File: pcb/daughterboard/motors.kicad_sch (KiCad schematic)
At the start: 20 parts, among them J10 Conn_01x06_Socket, J11 Conn_01x06_Socket, J12 Conn_01x06_Socket, J13 Conn_01x06_Socket, J14 Conn_01x06_Socket, J15 Conn_01x06_Socket, J16 Conn_01x06_Socket, J17 Conn_01x06_Socket, J18 Conn_01x06_Socket, J19 Conn_01x06_Socket, J20 Conn_01x06_Socket, J21 Conn_01x06_Socket, J22 Conn_01x06_Socket, J3 Conn_01x06_Socket, J4 Conn_01x06_Socket, J5 Conn_01x06_Socket, J6 Conn_01x06_Socket, J7 Conn_01x06_Socket, J8 Conn_01x06_Socket, J9 Conn_01x06_Socket

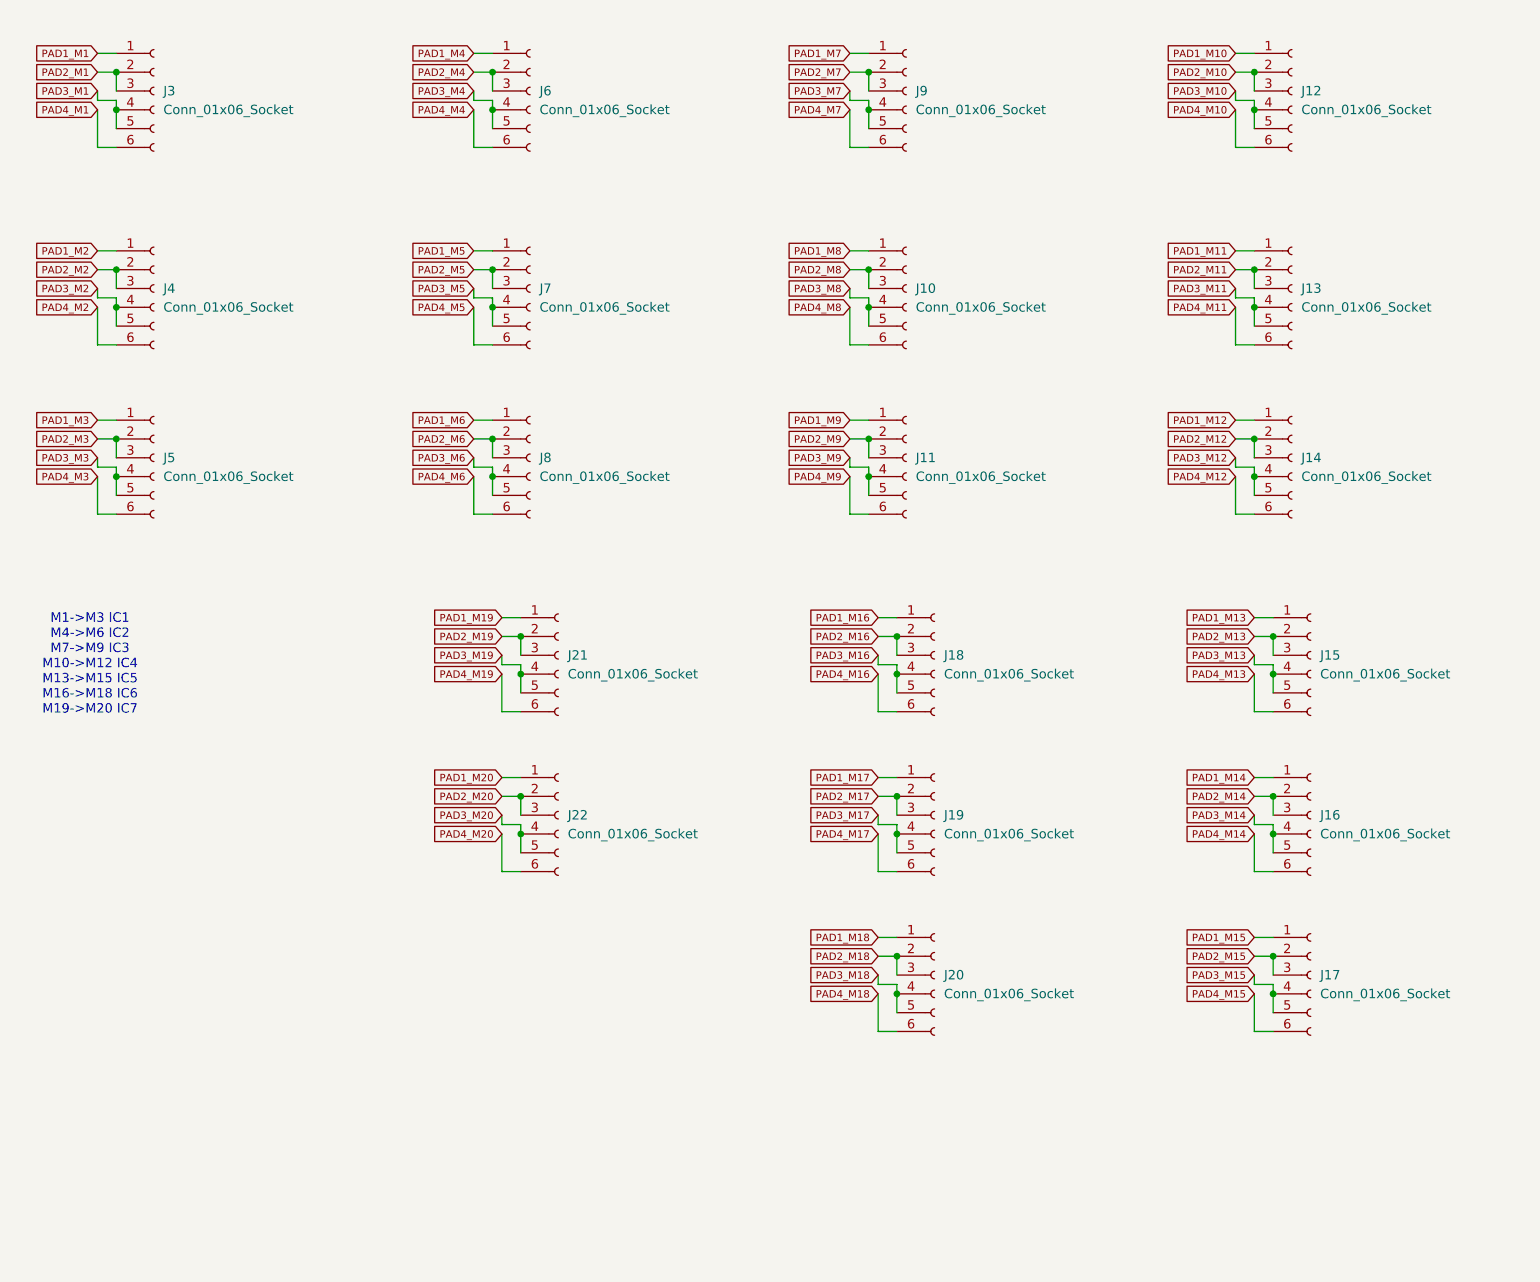
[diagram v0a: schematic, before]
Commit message: modified motor connectors
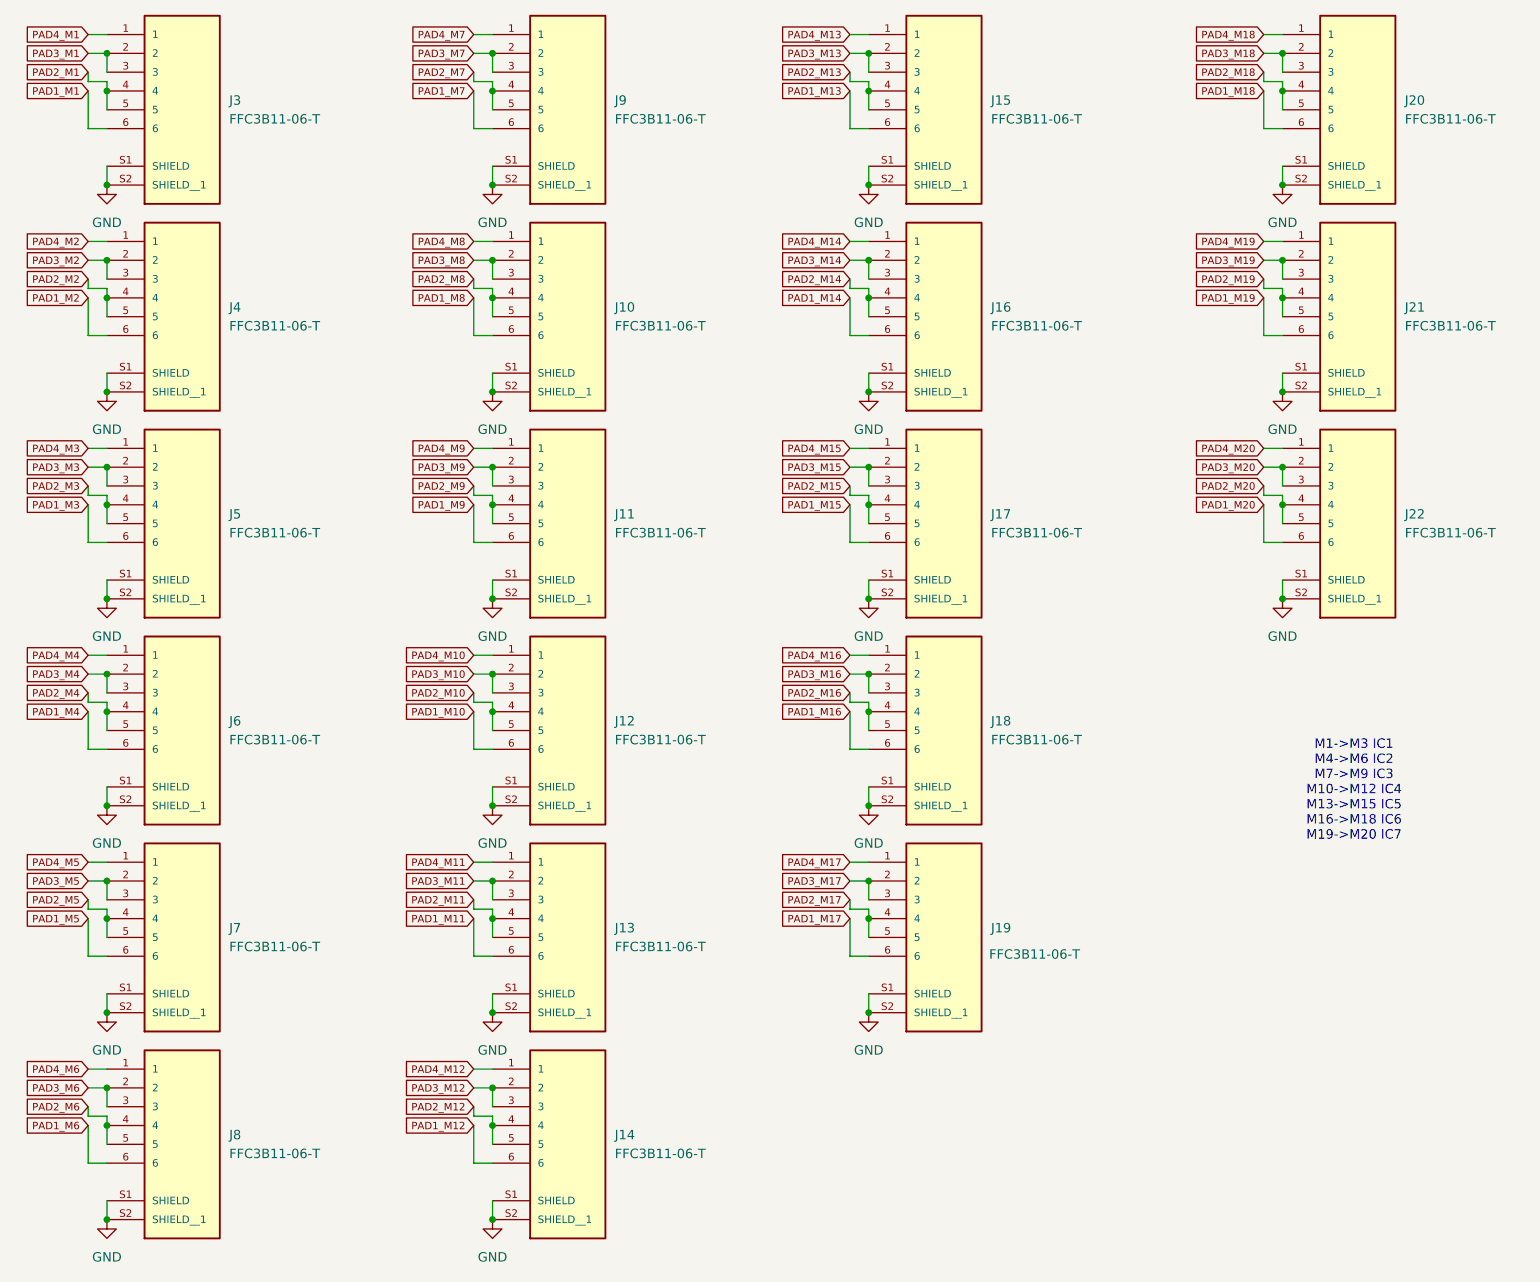
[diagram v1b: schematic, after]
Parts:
- removed J10, J11, J12, J13, J14, J15, J16, J17, J18, J19, J20, J21, J22, J3, J4, J5, J6, J7, J8, J9: Conn_01x06_Socket, 52207-0633:52207-0633, symbol Connector:Conn_01x06_Socket
- added J10, J11, J12, J13, J14, J15, J16, J17, J18, J19, J20, J21, J22, J3, J4, J5, J6, J7, J8, J9: FFC3B11-06-T, FFC3B11_06_T:GCT_FFC3B11-06-T, symbol FFC3B11-06-T:FFC3B11-06-T
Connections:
- net PAD1_M1: now also J3.6
- net PAD1_M10: now also J12.6
- net PAD1_M11: now also J13.6
- net PAD1_M12: now also J14.6
- net PAD1_M13: now also J15.6
- net PAD1_M14: now also J16.6
- net PAD1_M15: now also J17.6
- net PAD1_M16: now also J18.6
- net PAD1_M17: now also J19.6
- net PAD1_M18: now also J20.6
- net PAD1_M19: now also J21.6
- net PAD1_M2: now also J4.6
- net PAD1_M20: now also J22.6
- net PAD1_M3: now also J5.6
- net PAD1_M4: now also J6.6
- net PAD1_M5: now also J7.6
- net PAD1_M6: now also J8.6
- net PAD1_M7: now also J9.6
- net PAD1_M8: now also J10.6
- net PAD1_M9: now also J11.6
- net PAD2_M1: now also J3.4, J3.5
- net PAD2_M10: now also J12.4, J12.5
- net PAD2_M11: now also J13.4, J13.5
- net PAD2_M12: now also J14.4, J14.5
- net PAD2_M13: now also J15.4, J15.5
- net PAD2_M14: now also J16.4, J16.5
- net PAD2_M15: now also J17.4, J17.5
- net PAD2_M16: now also J18.4, J18.5
- net PAD2_M17: now also J19.4, J19.5
- net PAD2_M18: now also J20.4, J20.5
- net PAD2_M19: now also J21.4, J21.5
- net PAD2_M2: now also J4.4, J4.5
- net PAD2_M20: now also J22.4, J22.5
- net PAD2_M3: now also J5.4, J5.5
- net PAD2_M4: now also J6.4, J6.5
- net PAD2_M5: now also J7.4, J7.5
- net PAD2_M6: now also J8.4, J8.5
- net PAD2_M7: now also J9.4, J9.5
- net PAD2_M8: now also J10.4, J10.5
- net PAD2_M9: now also J11.4, J11.5
- net PAD3_M1: now also J3.2, J3.3
- net PAD3_M10: now also J12.2, J12.3
- net PAD3_M11: now also J13.2, J13.3
- net PAD3_M12: now also J14.2, J14.3
- net PAD3_M13: now also J15.2, J15.3
- net PAD3_M14: now also J16.2, J16.3
- net PAD3_M15: now also J17.2, J17.3
- net PAD3_M16: now also J18.2, J18.3
- net PAD3_M17: now also J19.2, J19.3
- net PAD3_M18: now also J20.2, J20.3
- net PAD3_M19: now also J21.2, J21.3
- net PAD3_M2: now also J4.2, J4.3
- net PAD3_M20: now also J22.2, J22.3
- net PAD3_M3: now also J5.2, J5.3
- net PAD3_M4: now also J6.2, J6.3
- net PAD3_M5: now also J7.2, J7.3
- net PAD3_M6: now also J8.2, J8.3
- net PAD3_M7: now also J9.2, J9.3
- net PAD3_M8: now also J10.2, J10.3
- net PAD3_M9: now also J11.2, J11.3
- net PAD4_M1: now also J3.1
- net PAD4_M10: now also J12.1
- net PAD4_M11: now also J13.1
- net PAD4_M12: now also J14.1
- net PAD4_M13: now also J15.1
- net PAD4_M14: now also J16.1
- net PAD4_M15: now also J17.1
- net PAD4_M16: now also J18.1
- net PAD4_M17: now also J19.1
- net PAD4_M18: now also J20.1
- net PAD4_M19: now also J21.1
- net PAD4_M2: now also J4.1
- net PAD4_M20: now also J22.1
- net PAD4_M3: now also J5.1
- net PAD4_M4: now also J6.1
- net PAD4_M5: now also J7.1
- net PAD4_M6: now also J8.1
- net PAD4_M7: now also J9.1
- net PAD4_M8: now also J10.1
- net PAD4_M9: now also J11.1
- new net GND: J10.S1 (SHIELD), J10.S2 (SHIELD__1), J11.S1 (SHIELD), J11.S2 (SHIELD__1), J12.S1 (SHIELD), J12.S2 (SHIELD__1), J13.S1 (SHIELD), J13.S2 (SHIELD__1), J14.S1 (SHIELD), J14.S2 (SHIELD__1), J15.S1 (SHIELD), J15.S2 (SHIELD__1), J16.S1 (SHIELD), J16.S2 (SHIELD__1), J17.S1 (SHIELD), J17.S2 (SHIELD__1), J18.S1 (SHIELD), J18.S2 (SHIELD__1), J19.S1 (SHIELD), J19.S2 (SHIELD__1), J20.S1 (SHIELD), J20.S2 (SHIELD__1), J21.S1 (SHIELD), J21.S2 (SHIELD__1), J22.S1 (SHIELD), J22.S2 (SHIELD__1), J3.S1 (SHIELD), J3.S2 (SHIELD__1), J4.S1 (SHIELD), J4.S2 (SHIELD__1), J5.S1 (SHIELD), J5.S2 (SHIELD__1), J6.S1 (SHIELD), J6.S2 (SHIELD__1), J7.S1 (SHIELD), J7.S2 (SHIELD__1), J8.S1 (SHIELD), J8.S2 (SHIELD__1), J9.S1 (SHIELD), J9.S2 (SHIELD__1)

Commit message: modified MPN
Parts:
- J10, J11, J12, J13, J14, J15, J16, J17, J18, J19, J20, J21, J22, J3, J4, J5, J6, J7, J8, J9: Manufacturer_Part_Number (none) -> FFC3B11-06-T
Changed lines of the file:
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@@
 			)
 		)
+		(property "Manufacturer_Part_Number" "FFC3B11-06-T"
+			(at 99.06 171.45 0)
+			(hide yes)
+			(show_name no)
+			(do_not_autoplace no)
+			(effects
+				(font
+					(size 1.27 1.27)
+				)
+			)
+		)
 		(pin "S2"
 		)
@@
 			)
 		)
+		(property "Manufacturer_Part_Number" "FFC3B11-06-T"
+			(at 205.74 59.69 0)
+			(hide yes)
+			(show_name no)
+			(do_not_autoplace no)
+			(effects
+				(font
+					(size 1.27 1.27)
+				)
+			)
+		)
 		(pin "S2"
 		)
@@
 			)
 		)
+		(property "Manufacturer_Part_Number" "FFC3B11-06-T"
+			(at 205.74 87.63 0)
+			(hide yes)
+			(show_name no)
+			(do_not_autoplace no)
+			(effects
+				(font
+					(size 1.27 1.27)
+				)
+			)
+		)
 		(pin "S2"
 		)
@@
 			)
 		)
+		(property "Manufacturer_Part_Number" "FFC3B11-06-T"
+			(at 99.06 59.69 0)
+			(hide yes)
+			(show_name no)
+			(do_not_autoplace no)
+			(effects
+				(font
+					(size 1.27 1.27)
+				)
+			)
+		)
 		(pin "S2"
 		)
@@
 			)
 		)
+		(property "Manufacturer_Part_Number" "FFC3B11-06-T"
+			(at 46.99 143.51 0)
+			(hide yes)
+			(show_name no)
+			(do_not_autoplace no)
+			(effects
+				(font
+					(size 1.27 1.27)
+				)
+			)
+		)
 		(pin "S2"
 		)
@@
 			)
 		)
+		(property "Manufacturer_Part_Number" "FFC3B11-06-T"
+			(at 205.74 31.75 0)
+			(hide yes)
+			(show_name no)
+			(do_not_autoplace no)
+			(effects
+				(font
+					(size 1.27 1.27)
+				)
+			)
+		)
 		(pin "S2"
 		)
@@
 			)
 		)
+		(property "Manufacturer_Part_Number" "FFC3B11-06-T"
+			(at 149.86 115.57 0)
+			(hide yes)
+			(show_name no)
+			(do_not_autoplace no)
+			(effects
+				(font
+					(size 1.27 1.27)
+				)
+			)
+		)
 		(pin "S2"
 		)
@@
 			)
 		)
+		(property "Manufacturer_Part_Number" "FFC3B11-06-T"
+			(at 99.06 87.63 0)
+			(hide yes)
+			(show_name no)
+			(do_not_autoplace no)
+			(effects
+				(font
+					(size 1.27 1.27)
+				)
+			)
+		)
 		(pin "S2"
 		)
@@
 			)
 		)
+		(property "Manufacturer_Part_Number" "FFC3B11-06-T"
+			(at 46.99 87.63 0)
+			(hide yes)
+			(show_name no)
+			(do_not_autoplace no)
+			(effects
+				(font
+					(size 1.27 1.27)
+				)
+			)
+		)
 		(pin "S2"
 		)
@@
 			)
 		)
+		(property "Manufacturer_Part_Number" "FFC3B11-06-T"
+			(at 46.99 115.57 0)
+			(hide yes)
+			(show_name no)
+			(do_not_autoplace no)
+			(effects
+				(font
+					(size 1.27 1.27)
+				)
+			)
+		)
 		(pin "S2"
 		)
@@
 			)
 		)
+		(property "Manufacturer_Part_Number" "FFC3B11-06-T"
+			(at 99.06 31.75 0)
+			(hide yes)
+			(show_name no)
+			(do_not_autoplace no)
+			(effects
+				(font
+					(size 1.27 1.27)
+				)
+			)
+		)
 		(pin "S2"
 		)
@@
 			)
 		)
+		(property "Manufacturer_Part_Number" "FFC3B11-06-T"
+			(at 46.99 31.75 0)
+			(hide yes)
+			(show_name no)
+			(do_not_autoplace no)
+			(effects
+				(font
+					(size 1.27 1.27)
+				)
+			)
+		)
 		(pin "S2"
 		)
@@
 			)
 		)
+		(property "Manufacturer_Part_Number" "FFC3B11-06-T"
+			(at 149.86 143.51 0)
+			(hide yes)
+			(show_name no)
+			(do_not_autoplace no)
+			(effects
+				(font
+					(size 1.27 1.27)
+				)
+			)
+		)
 		(pin "S2"
 		)
@@
 			)
 		)
+		(property "Manufacturer_Part_Number" "FFC3B11-06-T"
+			(at 149.86 59.69 0)
+			(hide yes)
+			(show_name no)
+			(do_not_autoplace no)
+			(effects
+				(font
+					(size 1.27 1.27)
+				)
+			)
+		)
 		(pin "S2"
 		)
@@
 			)
 		)
+		(property "Manufacturer_Part_Number" "FFC3B11-06-T"
+			(at 149.86 87.63 0)
+			(hide yes)
+			(show_name no)
+			(do_not_autoplace no)
+			(effects
+				(font
+					(size 1.27 1.27)
+				)
+			)
+		)
 		(pin "S2"
 		)
@@
 			)
 		)
+		(property "Manufacturer_Part_Number" "FFC3B11-06-T"
+			(at 99.06 115.57 0)
+			(hide yes)
+			(show_name no)
+			(do_not_autoplace no)
+			(effects
+				(font
+					(size 1.27 1.27)
+				)
+			)
+		)
 		(pin "S2"
 		)
@@
 			)
 		)
+		(property "Manufacturer_Part_Number" "FFC3B11-06-T"
+			(at 149.86 31.75 0)
+			(hide yes)
+			(show_name no)
+			(do_not_autoplace no)
+			(effects
+				(font
+					(size 1.27 1.27)
+				)
+			)
+		)
 		(pin "S2"
 		)
@@
 			)
 		)
+		(property "Manufacturer_Part_Number" "FFC3B11-06-T"
+			(at 46.99 171.45 0)
+			(hide yes)
+			(show_name no)
+			(do_not_autoplace no)
+			(effects
+				(font
+					(size 1.27 1.27)
+				)
+			)
+		)
 		(pin "S2"
 		)
@@
 			)
 		)
+		(property "Manufacturer_Part_Number" "FFC3B11-06-T"
+			(at 99.06 143.51 0)
+			(hide yes)
+			(show_name no)
+			(do_not_autoplace no)
+			(effects
+				(font
+					(size 1.27 1.27)
+				)
+			)
+		)
 		(pin "S2"
 		)
@@
 			)
 		)
+		(property "Manufacturer_Part_Number" "FFC3B11-06-T"
+			(at 46.99 59.69 0)
+			(hide yes)
+			(show_name no)
+			(do_not_autoplace no)
+			(effects
+				(font
+					(size 1.27 1.27)
+				)
+			)
+		)
